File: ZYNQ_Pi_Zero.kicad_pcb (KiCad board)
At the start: 4 copper layers, 33 parts, among them Q501 2N7002, Q502 2N7002, Q503 2N7002, U101 xc7z010clg400, U201 MT41K256M16TW-107_P, U301 W25Q256FVEI, U501 TPD4E05U06DQA, U502 TPD4E05U06DQA

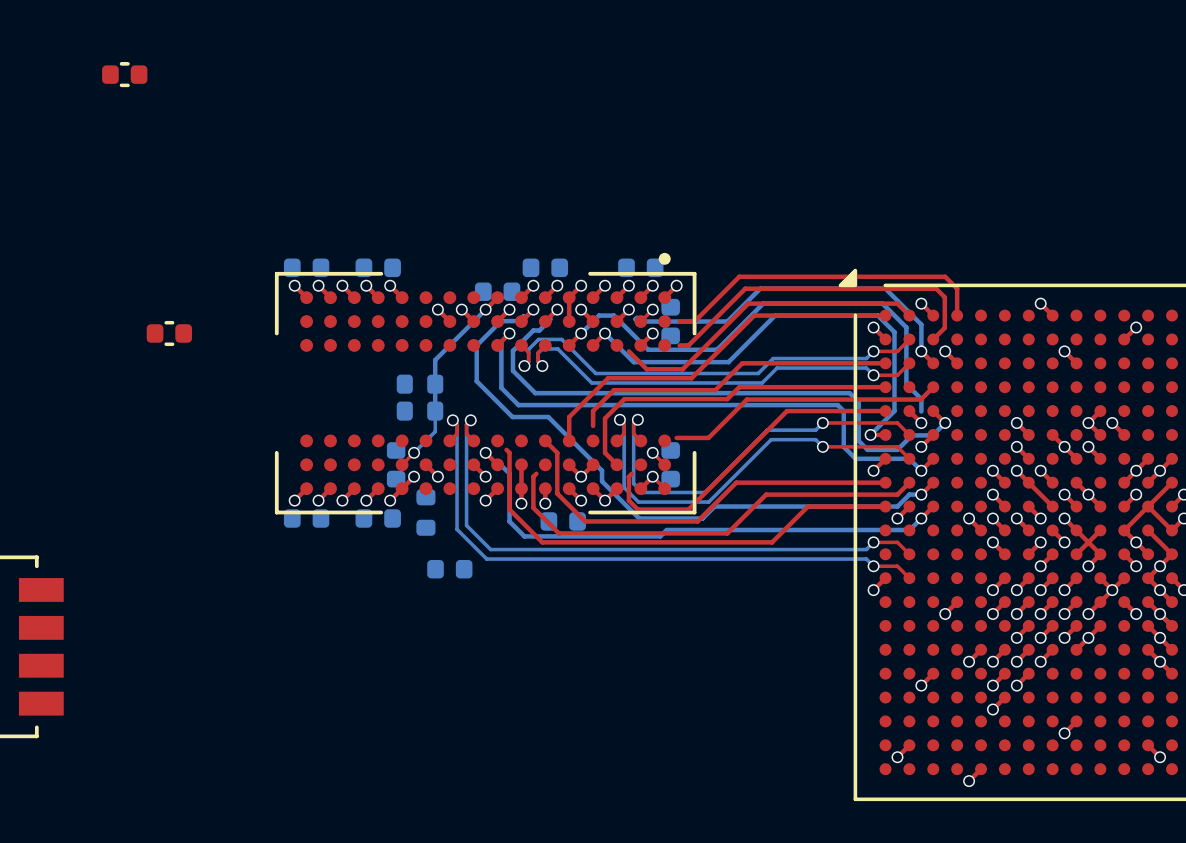
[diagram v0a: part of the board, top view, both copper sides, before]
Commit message: feat: continue routing dd3
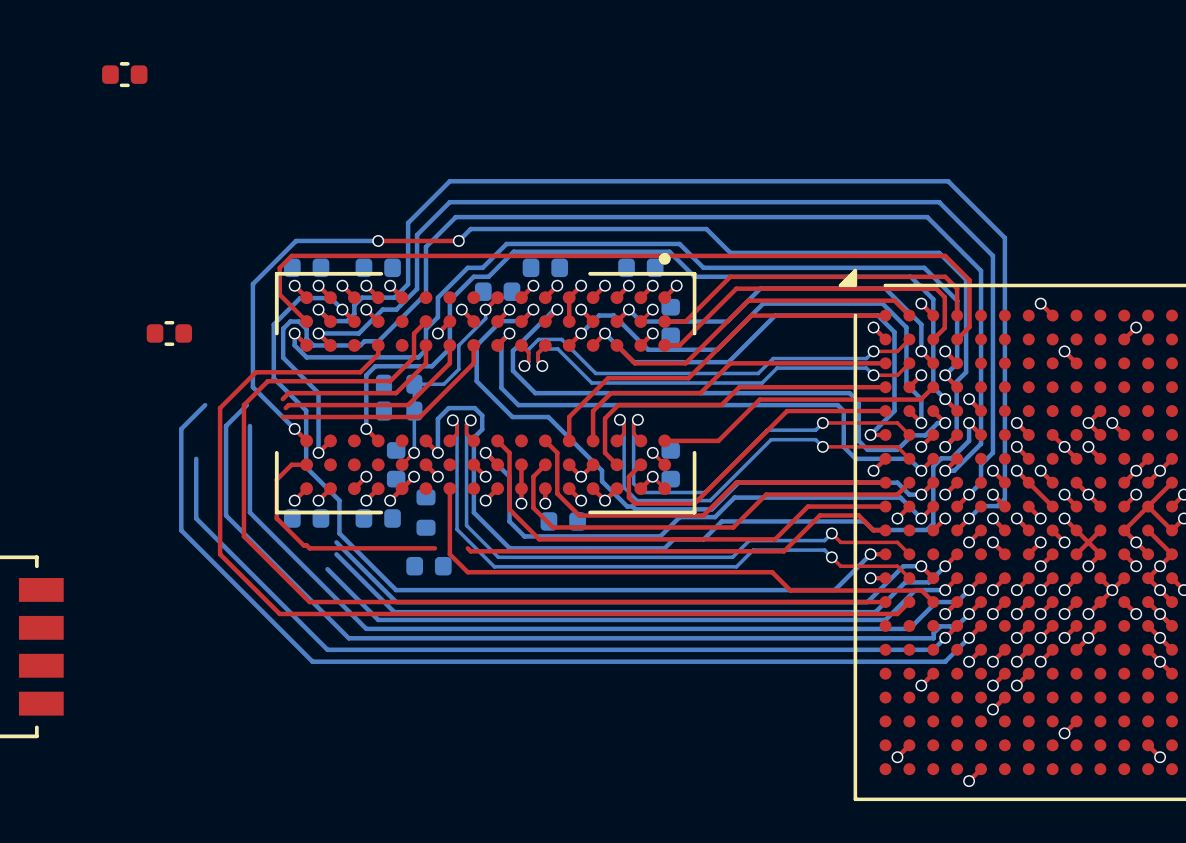
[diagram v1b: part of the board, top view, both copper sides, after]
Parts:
- moved C210 0.71 mm to (126.1, 100.8)
- moved R202 0.70 mm to (125.1, 95.6)
- moved R203 0.70 mm to (125.1, 94.7)
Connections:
- U201 pad A2: /DDR3/DDR_D2 -> /DDR3/DDR_D3
- U201 pad A3: /DDR3/DDR_D0 -> /DDR3/DDR_D1
- U201 pad A7: /DDR3/DDR_D3 -> /DDR3/DDR_D4
- U201 pad B8: /DDR3/DDR_D1 -> /DDR3/DDR_D7
- U201 pad C2: /DDR3/DDR_D4 -> /DDR3/DDR_D0
- U201 pad C3: /DDR3/DDR_D6 -> /DDR3/DDR_D2
- U201 pad D7: /DDR3/DDR_D7 -> /DDR3/DDR_D6
- U201 pad E3: /DDR3/DDR_D15 -> /DDR3/DDR_D8
- U201 pad F2: /DDR3/DDR_D13 -> /DDR3/DDR_D9
- U201 pad F8: /DDR3/DDR_D12 -> /DDR3/DDR_D13
- U201 pad G2: /DDR3/DDR_D9 -> /DDR3/DDR_D11
- U201 pad H3: /DDR3/DDR_D11 -> /DDR3/DDR_D10
- U201 pad H7: /DDR3/DDR_D8 -> /DDR3/DDR_D15
- U201 pad H8: /DDR3/DDR_D10 -> /DDR3/DDR_D12
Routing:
- net /DDR3/DDR_A11: track 0.00 -> 40.6 mm, vias 0 -> 2
- net /DDR3/DDR_~{CAS}: track 0.00 -> 40.4 mm, vias 0 -> 1
- net /DDR3/DDR_A7: track 0.00 -> 38.6 mm, vias 0 -> 2
- net /DDR3/DDR_A14: track 0.00 -> 37.8 mm, vias 0 -> 4
- net /DDR3/DDR_~{RAS}: track 0.00 -> 37.4 mm, vias 0 -> 1
- net /DDR3/DDR_A9: track 0.00 -> 35.7 mm, vias 0 -> 2
- net /DDR3/DDR_~{WE}: track 0.00 -> 35.6 mm, vias 0 -> 1
- net /DDR3/DDR_A0: track 0.00 -> 35.3 mm
- net /DDR3/DDR_~{CS}: track 0.00 -> 34.5 mm
- net /DDR3/DDR_ODT: track 0.00 -> 31.7 mm, vias 0 -> 1
- net /DDR3/DDR_A5: track 0.00 -> 30.9 mm, vias 0 -> 2
- net /DDR3/DDR_A13: track 0.00 -> 29.7 mm, vias 0 -> 2
- net /DDR3/DDR_A12: track 0.00 -> 28.8 mm, vias 0 -> 2
- net /DDR3/DDR_~{RESET}: track 0.00 -> 27.9 mm
- net /DDR3/DDR_A10: track 0.00 -> 27.9 mm, vias 0 -> 2
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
